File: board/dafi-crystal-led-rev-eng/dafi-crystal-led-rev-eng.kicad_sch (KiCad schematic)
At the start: 19 parts, among them SW1 SW_DPST_x2, U1 STM8L051F3P, U2 LIS2DW12

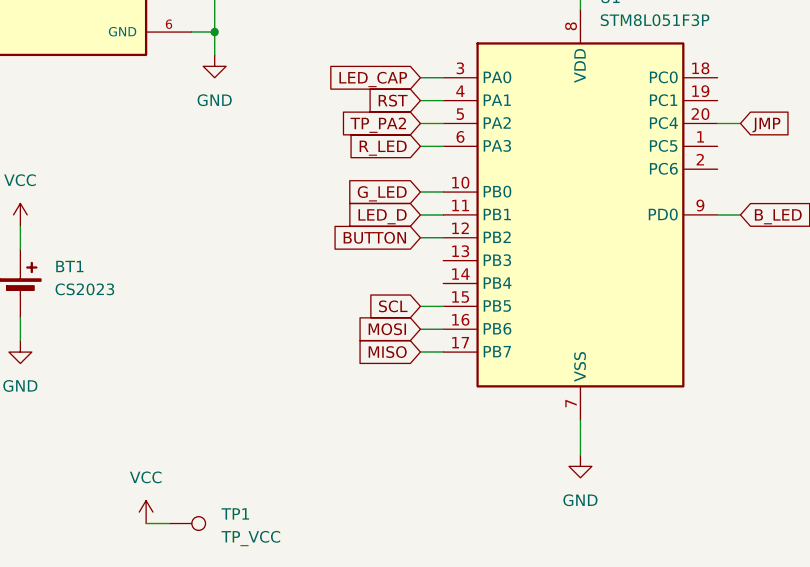
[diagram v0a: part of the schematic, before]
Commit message: messing around with uart
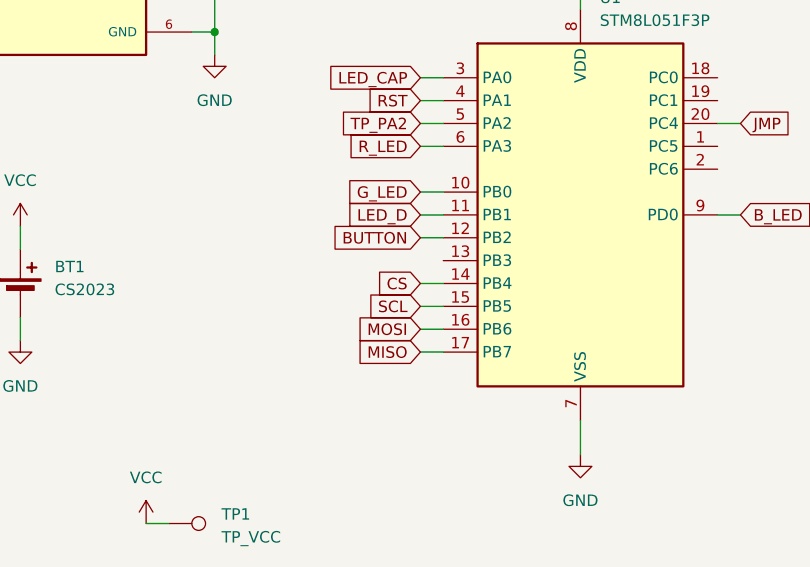
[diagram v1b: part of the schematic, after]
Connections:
- net CS: now also U1.14 (PB4)
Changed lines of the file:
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@@
+	(wire
+		(pts
+			(xy 123.19 105.41) (xy 125.73 105.41)
+		)
+		(stroke
+			(width 0)
+			(type default)
+		)
+	)
 	(wire
 		(pts
@@
 			(effects
 				(font
+					(size 1.27 1.27)
+				)
+				(justify right)
+				(hide yes)
+			)
+		)
+	)
+	(global_label "CS"
+		(shape input)
+		(at 123.19 105.41 180)
+		(fields_autoplaced yes)
+		(effects
+			(font
+				(size 1.27 1.27)
+			)
+			(justify right)
+		)
+		(property "Intersheetrefs" "${INTERSHEET_REFS}"
+			(at 117.7253 105.41 0)
+			(effects
+				(font
